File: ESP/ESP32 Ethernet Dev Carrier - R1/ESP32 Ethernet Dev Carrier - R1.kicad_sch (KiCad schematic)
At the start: 49 parts, among them J10 Conn_01x09, J11 Conn_01x04, J12 Conn_01x04, J13 Conn_01x04, J14 Conn_01x04, J3 ESP32-DevBoard-Header, J4 Conn_01x05, J5 Conn_01x05, J6 Conn_01x05, J7 Conn_01x09, J8 Conn_01x09, J9 Conn_01x09, SW1 SW_Push, U1 ESP32-WROVER-B_(16MB)

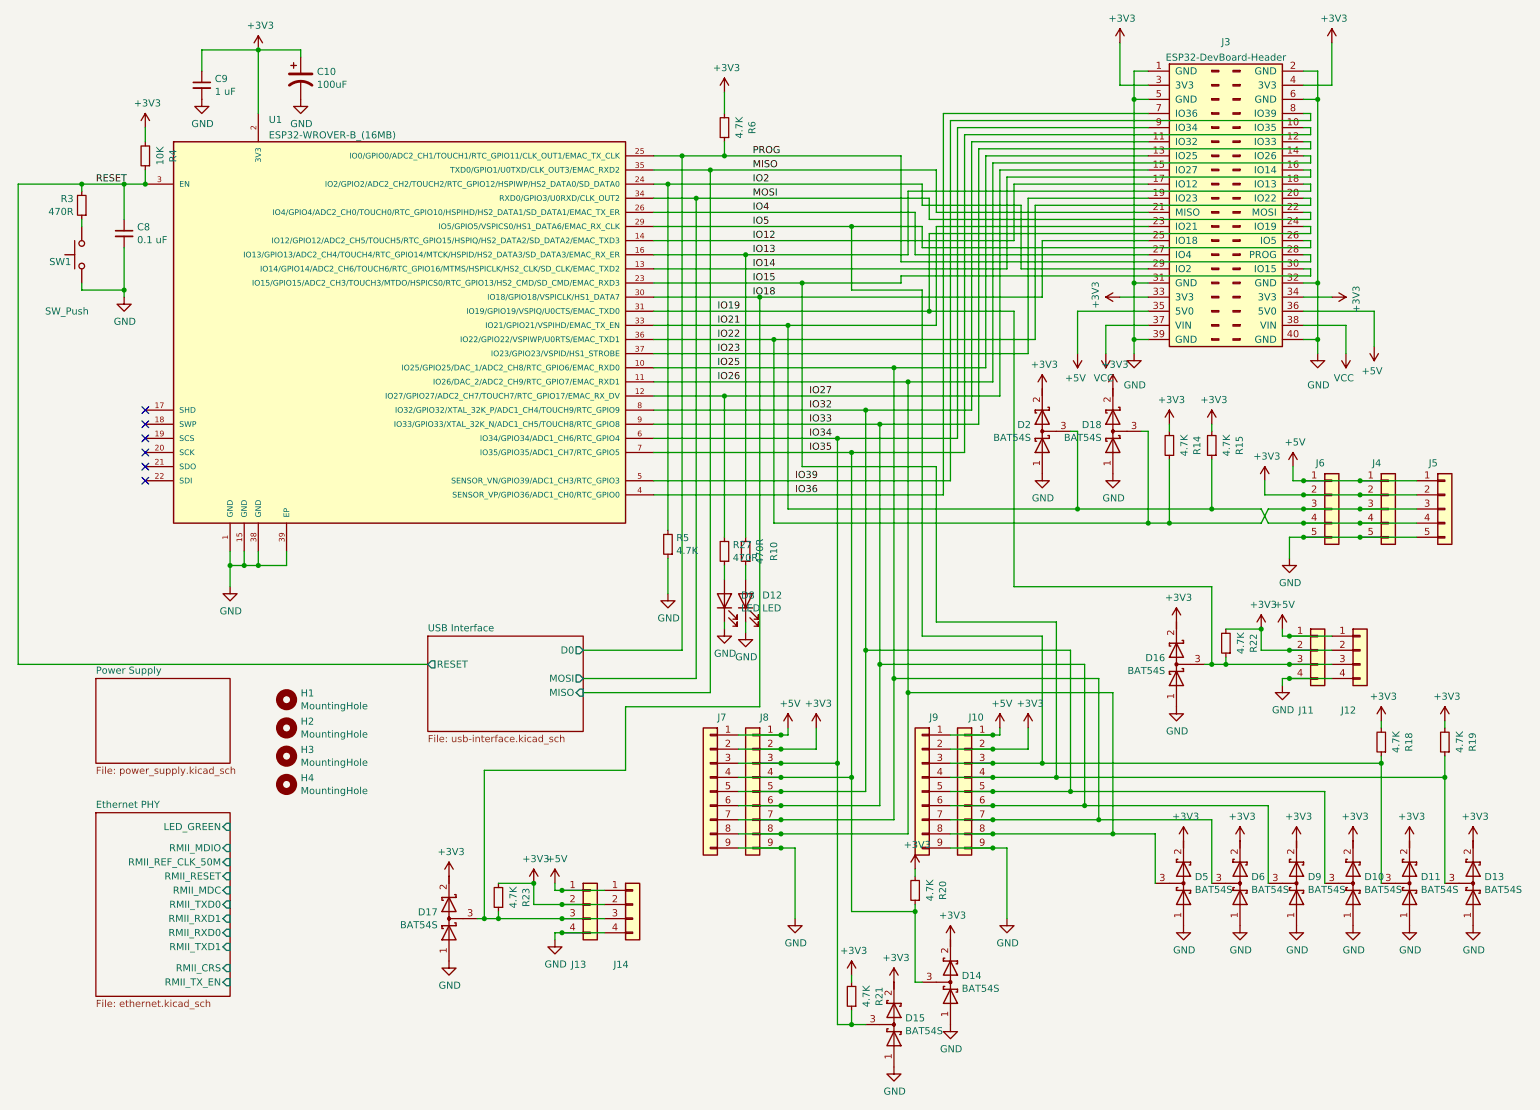
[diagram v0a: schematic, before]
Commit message: More work.
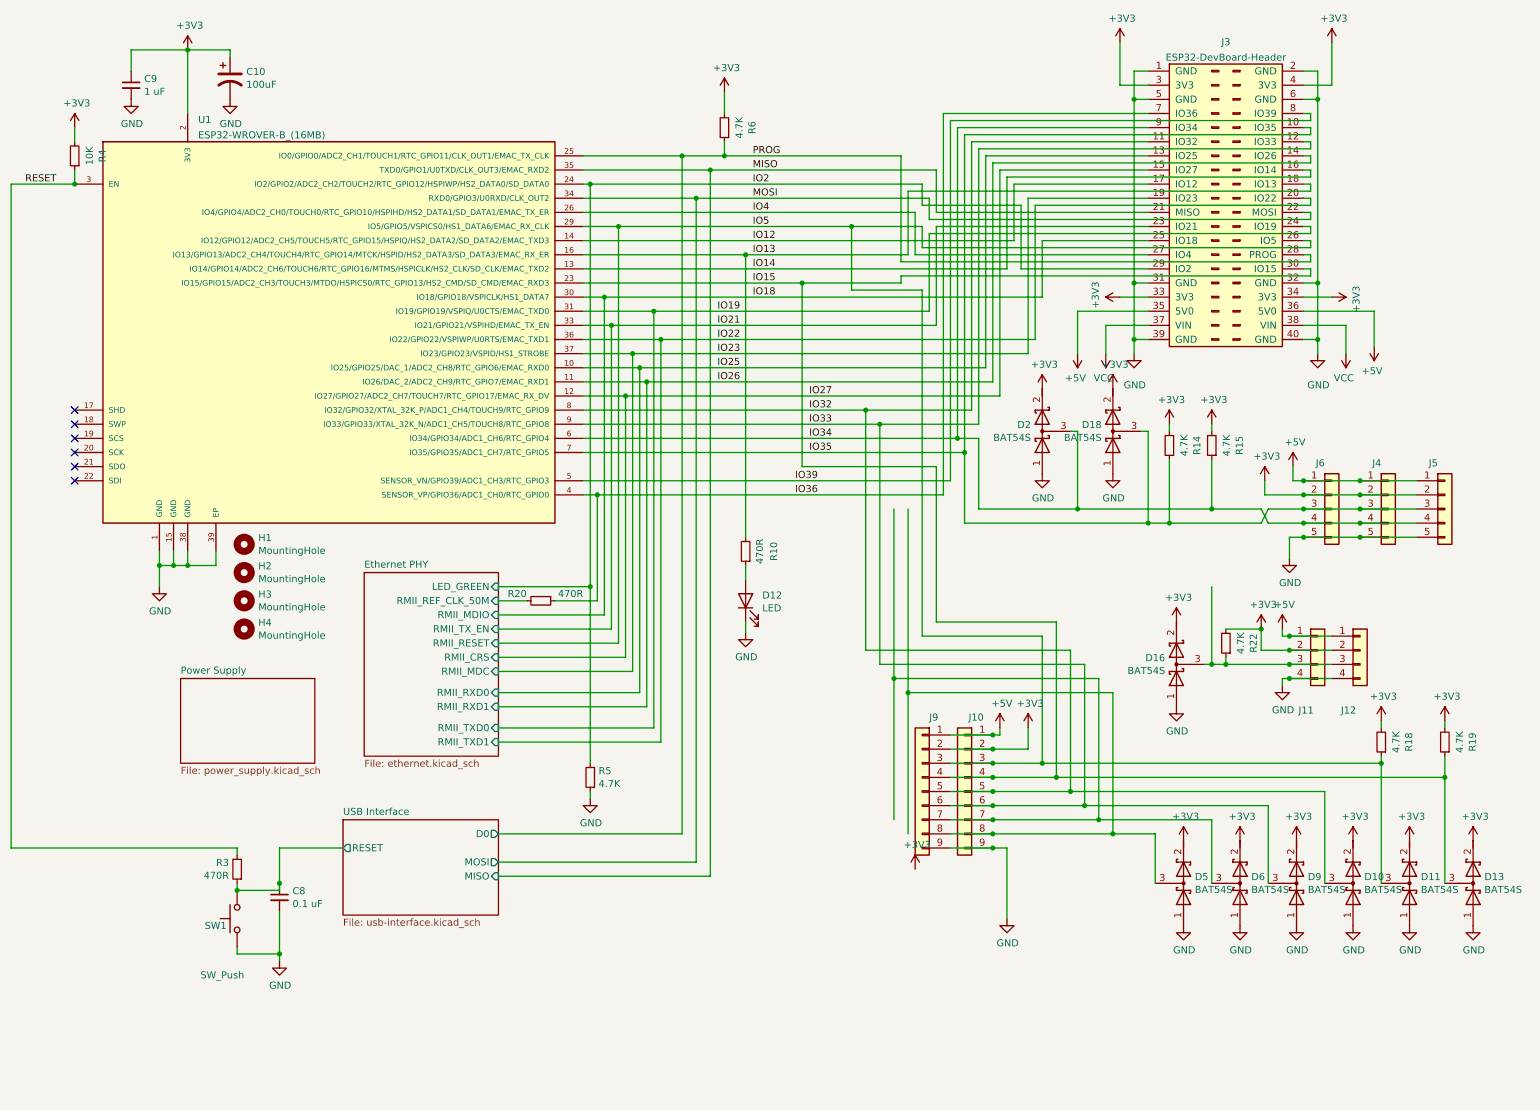
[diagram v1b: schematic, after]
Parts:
- removed D14, D15: BAT54S, Package_TO_SOT_SMD:SOT-23, symbol ESP32-Water-Meter-Monitor-rescue:D_Schottky_x2_Serial_AKC-Device
- removed D17: BAT54S, Package_TO_SOT_SMD:SOT-23, symbol Device:D_Schottky_x2_Serial_AKC
- removed D8: LED, custom:CHIPLED_0603, symbol Device:LED
- removed J13, J14: Conn_01x04, Connector_JST:JST_XH_B4B-XH-A_1x04_P2.50mm_Vertical, symbol Connector_Generic:Conn_01x04
- removed J7, J8: Conn_01x09, Connector_JST:JST_XH_B9B-XH-A_1x09_P2.50mm_Vertical, symbol Connector_Generic:Conn_01x09
- removed R21, R23: 4.7K, Resistor_SMD:R_0603_1608Metric, symbol Device:R_Small
- removed R27: 470R, Resistor_SMD:R_0603_1608Metric, symbol Device:R_Small
- R20: value 4.7K -> 470R
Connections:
- net +3V3: no longer R20.2
- net Ethernet PHY/RMII_REF_CLK_50M: now also R20.2
- net IO19: no longer D16.3 (common), J11.3 (Pin_3), J12.3 (Pin_3), R22.1
- net IO21: no longer D2.3 (common), J4.4 (Pin_4), J5.4 (Pin_4), J6.4 (Pin_4), R15.1
- net IO22: no longer D18.3 (common), J4.3 (Pin_3), J5.3 (Pin_3), J6.3 (Pin_3), R14.1
- net IO25: no longer D6.3 (common), J10.7 (Pin_7), J9.7 (Pin_7)
- net IO26: no longer D5.3 (common), J10.8 (Pin_8), J9.8 (Pin_8)
- net IO34: now also D2.3 (common), J4.4 (Pin_4), J5.4 (Pin_4), J6.4 (Pin_4), R15.1
- net IO35: now also D18.3 (common), J4.3 (Pin_3), J5.3 (Pin_3), J6.3 (Pin_3), R14.1; no longer R20.1
- net IO36: now also R20.1
- net RESET: no longer C8.1
- net USB Interface/RESET: now reaches R3.1, SW1.1
- net USB Interface/RESET: now also C8.1
- new net: D16.3 (common), J11.3 (Pin_3), J12.3 (Pin_3), R22.1
- new net: D6.3 (common), J10.7 (Pin_7), J9.7 (Pin_7)
- new net: D5.3 (common), J10.8 (Pin_8), J9.8 (Pin_8)
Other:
- moved on the sheet: C10, C8, C9, H1, H2, H3, H4, R3, R4, R5, SW1, U1
